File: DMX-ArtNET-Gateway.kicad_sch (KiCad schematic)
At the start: 45 parts, among them J1 GPIO Breakout, J2 DMX1, J3 DMX2, J4 Barrel_Jack_MountingPin, U1 AMS1117-3.3, U2 ESP32-WROOM-32D, U3 MAX485CSA, U4 MAX485CSA

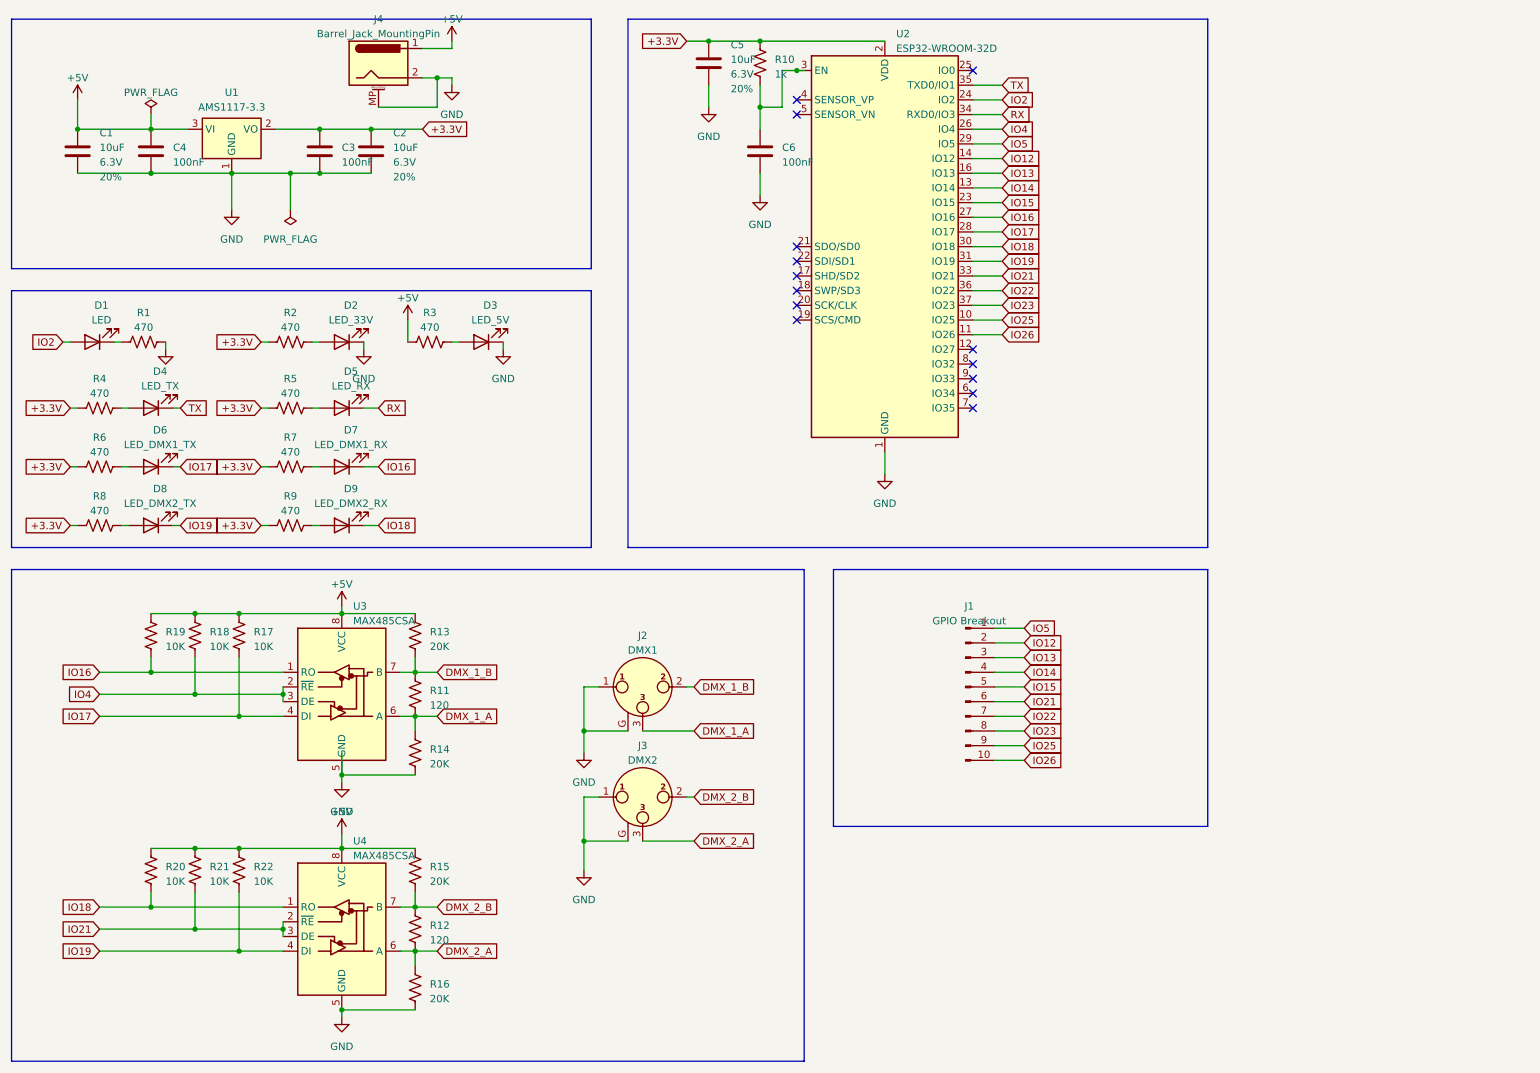
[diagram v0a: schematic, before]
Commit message: Firmware checkin
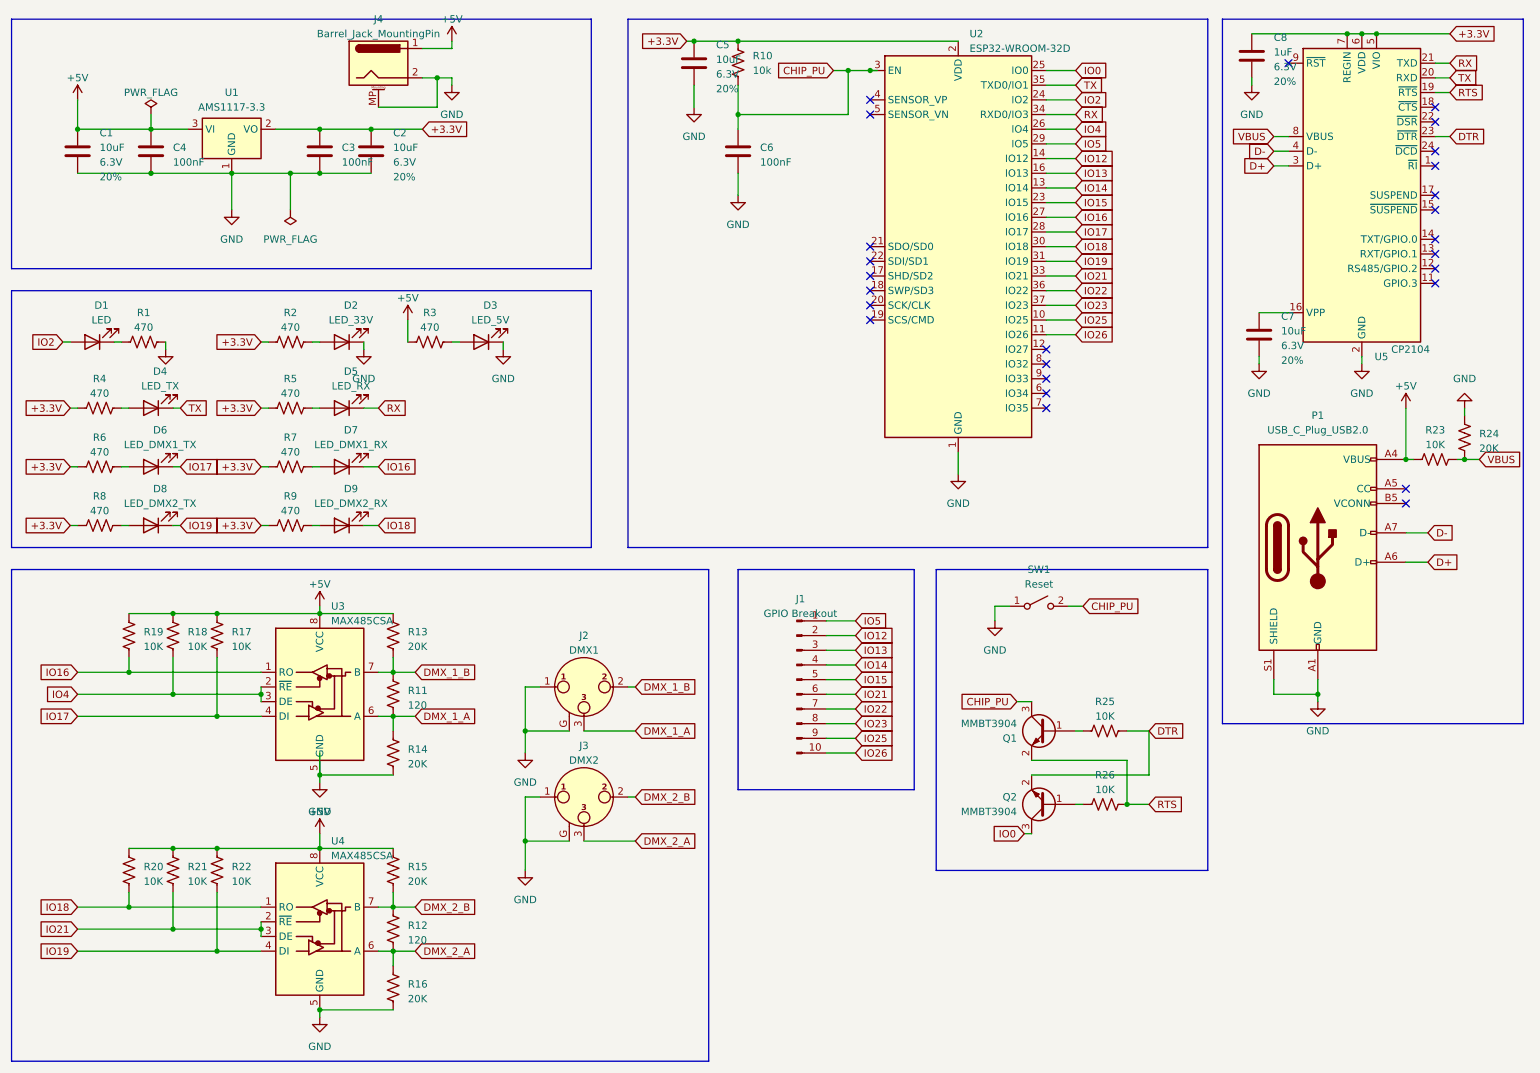
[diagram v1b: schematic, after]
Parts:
- added C7: 10uF, Capacitor_SMD:CP_Elec_3x5.3, symbol SparkFun-Capacitor:10uF_0603_6.3V_20%
- added C8: 1uF, Capacitor_SMD:CP_Elec_3x5.3, symbol SparkFun-Capacitor:10uF_0603_6.3V_20%
- added P1: USB_C_Plug_USB2.0, Connector_USB:USB_C_Receptacle_GCT_USB4105-xx-A_16P_TopMnt_Horizontal, symbol Connector:USB_C_Plug_USB2.0
- added Q1, Q2: MMBT3904, Package_TO_SOT_SMD:SOT-23, symbol Transistor_BJT:MMBT3904
- added R23, R25, R26: 10K, SparkFun-Resistor:R_0805_2012Metric, symbol SparkFun-Resistor:R
- added R24: 20K, SparkFun-Resistor:R_0805_2012Metric, symbol SparkFun-Resistor:R
- added SW1: Reset, SparkFun-Switch:Momentary_SMD_4.6x2.8mm, symbol SparkFun-Switch:SPST_Momentary_4.6x2.8mm
- added U5: CP2104, Package_DFN_QFN:QFN-24-1EP_4x4mm_P0.5mm_EP2.6x2.6mm, symbol Interface_USB:CP2104
- R10: value 1k -> 10k
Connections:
- net +3.3V: now also C8.1, U5.5 (VIO), U5.6 (VDD), U5.7 (REGIN)
- net +5V: now also P1.A4 (VBUS), P1.A9 (VBUS), P1.B4 (VBUS), P1.B9 (VBUS), R23.1
- net GND: now also C7.2, C8.2, P1.A1 (GND), P1.A12 (GND), P1.B1 (GND), P1.B12 (GND), P1.S1 (SHIELD), R24.1, SW1.1 (A), U5.2 (GND), U5.25 (GND)
- net RX: now also U5.21 (TXD)
- net TX: now also U5.20 (RXD)
- net CHIP_PU: now reaches C6.1, R10.2, U2.3 (EN)
- net CHIP_PU: now also Q1.3 (C), SW1.2 (B)
- net IO0: now reaches U2.25 (IO0)
- net IO0: now also Q2.3 (C)
- new net: Q1.1 (B), R25.1
- new net: C7.1, U5.16 (VPP)
- new net: Q2.1 (B), R26.1
- new net D+: P1.A6 (D+), U5.3 (D+)
- new net D-: P1.A7 (D-), U5.4 (D-)
- new net DTR: Q2.2 (E), R25.2, U5.23 (~{DTR})
- new net RTS: Q1.2 (E), R26.2, U5.19 (~{RTS})
- new net VBUS: R23.2, R24.2, U5.8 (VBUS)
- no-connect marks 14 -> 26
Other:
- moved on the sheet: C5, C6, J1, J2, J3, R10, R11, R12, R13, R14, R15, R16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
